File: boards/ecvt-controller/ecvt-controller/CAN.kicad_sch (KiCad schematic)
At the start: 23 parts, among them SW1 SW_SPST, SW2 SW_SPST, U1 TJA1051T-3, U3 MCP2515-xSO, U5 ACT45B-101-2P-TL003, U6 PESD2CAN,215, Y2 ABM3-16.000MHZ-D2Y-T

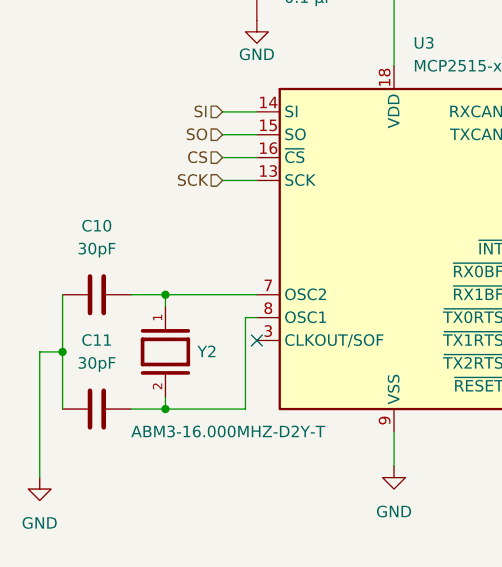
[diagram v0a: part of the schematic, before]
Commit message: ADC done
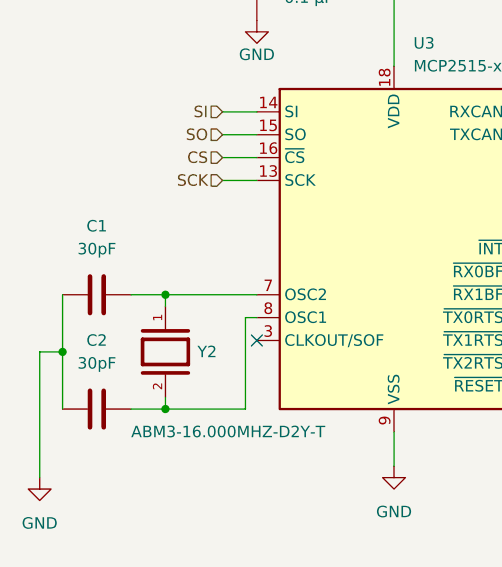
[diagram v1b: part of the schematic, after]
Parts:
- removed C10, C11: 30pF, Capacitor_SMD:C_0805_2012Metric_Pad1.18x1.45mm_HandSolder, symbol Device:C
- added C1, C2: 30pF, Capacitor_SMD:C_0603_1608Metric_Pad1.08x0.95mm_HandSolder, symbol baja-common-parts:C_0603
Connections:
- net GND: now also C1.1, C2.1
- net at U3.7 (OSC2), Y2.1: now also C1.2
- net at U3.8 (OSC1), Y2.2: now also C2.2
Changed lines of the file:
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@@
 			)
 		)
-		(property "Datasheet" ""
+		(property "Datasheet" "file://C:\\Users\\manas\\OneDrive - Northwestern University\\Northwestern\\Extracurricular\\hardware\\libraries\\datasheets\\cmf_automotive_signal_act45b_en.pdf"
 			(at 214.63 97.79 0)
 			(hide yes)
@@
 	)
 	(symbol
-		(lib_id "Device:C")
-		(at 21.59 124.46 90)
-		(unit 1)
-		(body_style 1)
-		(exclude_from_sim no)
-		(in_bom yes)
-		(on_board yes)
-		(in_pos_files yes)
-		(dnp no)
-		(fields_autoplaced yes)
-		(property "Reference" "C11"
-			(at 21.59 116.84 90)
-			(show_name no)
-			(do_not_autoplace no)
-			(effects
-				(font
-					(size 1.27 1.27)
-				)
-			)
-		)
-		(property "Value" "30pF"
-			(at 21.59 119.38 90)
-			(show_name no)
-			(do_not_autoplace no)
-			(effects
-				(font
-					(size 1.27 1.27)
-				)
-			)
-		)
-		(property "Footprint" "Capacitor_SMD:C_0805_2012Metric_Pad1.18x1.45mm_HandSolder"
-			(at 25.4 123.4948 0)
-			(hide yes)
-			(show_name no)
-			(do_not_autoplace no)
-			(effects
-				(font
-					(size 1.27 1.27)
-				)
-			)
-		)
-		(property "Datasheet" ""
-			(at 21.59 124.46 0)
-			(hide yes)
-			(show_name no)
-			(do_not_autoplace no)
-			(effects
-				(font
-					(size 1.27 1.27)
-				)
-			)
-		)
-		(property "Description" "Unpolarized capacitor"
-			(at 21.59 124.46 0)
-			(hide yes)
-			(show_name no)
-			(do_not_autoplace no)
-			(effects
-				(font
-					(size 1.27 1.27)
-				)
-			)
-		)
-		(pin "1"
-		)
-		(pin "2"
-		)
-		(instances
-			(project "ecvt-controller"
-				(path "/6a3c849d-efdf-47ab-8467-b82fc2fbc70f/577f7b7d-9ccb-4072-8b99-2d0e10acd900"
-					(reference "C11")
-					(unit 1)
-				)
-			)
-		)
-	)
-	(symbol
 		(lib_id "power:+3.3V")
 		(at 54.61 66.04 0)
@@
 			)
 		)
-		(property "Datasheet" ""
+		(property "Datasheet" "file://C:\\Users\\manas\\OneDrive - Northwestern University\\Northwestern\\Extracurricular\\hardware\\libraries\\datasheets\\PESD2CANFD24VT-Q.pdf"
 			(at 186.69 91.44 0)
 			(hide yes)
@@
 	)
 	(symbol
+		(lib_id "baja-common-parts:C_0603")
+		(at 21.59 124.46 90)
+		(unit 1)
+		(body_style 1)
+		(exclude_from_sim no)
+		(in_bom yes)
+		(on_board yes)
+		(in_pos_files yes)
+		(dnp no)
+		(fields_autoplaced yes)
+		(property "Reference" "C2"
+			(at 21.59 116.84 90)
+			(show_name no)
+			(do_not_autoplace no)
+			(effects
+				(font
+					(size 1.27 1.27)
+				)
+			)
+		)
+		(property "Value" "30pF"
+			(at 21.59 119.38 90)
+			(show_name no)
+			(do_not_autoplace no)
+			(effects
+				(font
+					(size 1.27 1.27)
+				)
+			)
+		)
+		(property "Footprint" "Capacitor_SMD:C_0603_1608Metric_Pad1.08x0.95mm_HandSolder"
+			(at 24.13 124.46 0)
+			(hide yes)
+			(show_name no)
+			(do_not_autoplace no)
+			(effects
+				(font
+					(size 1.27 1.27)
+				)
+			)
+		)
+		(property "Datasheet" ""
+			(at 26.67 124.46 0)
+			(hide yes)
+			(show_name no)
+			(do_not_autoplace no)
+			(effects
+				(font
+					(size 1.27 1.27)
+				)
+			)
+		)
+		(property "Description" "Capacitor 0603 (1608 metric) HandSolder - Baja default passive size"
+			(at 29.21 124.46 0)
+			(hide yes)
+			(show_name no)
+			(do_not_autoplace no)
+			(effects
+				(font
+					(size 1.27 1.27)
+				)
+			)
+		)
+		(pin "2"
+		)
+		(pin "1"
+		)
+		(instances
+			(project "ecvt-controller"
+				(path "/6a3c849d-efdf-47ab-8467-b82fc2fbc70f/577f7b7d-9ccb-4072-8b99-2d0e10acd900"
+					(reference "C2")
+					(unit 1)
+				)
+			)
+		)
+	)
+	(symbol
 		(lib_id "Device:C")
 		(at 269.24 123.19 0)
@@
 				(path "/6a3c849d-efdf-47ab-8467-b82fc2fbc70f/577f7b7d-9ccb-4072-8b99-2d0e10acd900"
 					(reference "#PWR049")
-					(unit 1)
-				)
-			)
-		)
-	)
-	(symbol
-		(lib_id "Device:C")
-		(at 21.59 111.76 90)
-		(unit 1)
-		(body_style 1)
-		(exclude_from_sim no)
-		(in_bom yes)
-		(on_board yes)
-		(in_pos_files yes)
-		(dnp no)
-		(fields_autoplaced yes)
-		(property "Reference" "C10"
-			(at 21.59 104.14 90)
-			(show_name no)
-			(do_not_autoplace no)
-			(effects
-				(font
-					(size 1.27 1.27)
-				)
-			)
-		)
-		(property "Value" "30pF"
-			(at 21.59 106.68 90)
-			(show_name no)
-			(do_not_autoplace no)
-			(effects
-				(font
-					(size 1.27 1.27)
-				)
-			)
-		)
-		(property "Footprint" "Capacitor_SMD:C_0805_2012Metric_Pad1.18x1.45mm_HandSolder"
-			(at 25.4 110.7948 0)
-			(hide yes)
-			(show_name no)
-			(do_not_autoplace no)
-			(effects
-				(font
-					(size 1.27 1.27)
-				)
-			)
-		)
-		(property "Datasheet" ""
-			(at 21.59 111.76 0)
-			(hide yes)
-			(show_name no)
-			(do_not_autoplace no)
-			(effects
-				(font
-					(size 1.27 1.27)
-				)
-			)
-		)
-		(property "Description" "Unpolarized capacitor"
-			(at 21.59 111.76 0)
-			(hide yes)
-			(show_name no)
-			(do_not_autoplace no)
-			(effects
-				(font
-					(size 1.27 1.27)
-				)
-			)
-		)
-		(pin "1"
-		)
-		(pin "2"
-		)
-		(instances
-			(project "ecvt-controller"
-				(path "/6a3c849d-efdf-47ab-8467-b82fc2fbc70f/577f7b7d-9ccb-4072-8b99-2d0e10acd900"
-					(reference "C10")
 					(unit 1)
 				)
@@
 					(unit 1)
 				)
+			)
+		)
+	)
+	(symbol
+		(lib_id "baja-common-parts:C_0603")
+		(at 21.59 111.76 90)
+		(unit 1)
+		(body_style 1)
+		(exclude_from_sim no)
+		(in_bom yes)
+		(on_board yes)
+		(in_pos_files yes)
+		(dnp no)
+		(fields_autoplaced yes)
+		(property "Reference" "C1"
+			(at 21.59 104.14 90)
+			(show_name no)
+			(do_not_autoplace no)
+			(effects
+				(font
+					(size 1.27 1.27)
+				)
+			)
+		)
+		(property "Value" "30pF"
+			(at 21.59 106.68 90)
+			(show_name no)
+			(do_not_autoplace no)
+			(effects
+				(font
+					(size 1.27 1.27)
+				)
+			)
+		)
+		(property "Footprint" "Capacitor_SMD:C_0603_1608Metric_Pad1.08x0.95mm_HandSolder"
+			(at 24.13 111.76 0)
+			(hide yes)
+			(show_name no)
+			(do_not_autoplace no)
+			(effects
+				(font
+					(size 1.27 1.27)
+				)
+			)
+		)
+		(property "Datasheet" ""
+			(at 26.67 111.76 0)
+			(hide yes)
+			(show_name no)
+			(do_not_autoplace no)
+			(effects
+				(font
+					(size 1.27 1.27)
+				)
+			)
+		)
+		(property "Description" "Capacitor 0603 (1608 metric) HandSolder - Baja default passive size"
+			(at 29.21 111.76 0)
+			(hide yes)
+			(show_name no)
+			(do_not_autoplace no)
+			(effects
+				(font
+					(size 1.27 1.27)
+				)
+			)
+		)
+		(pin "2"
+		)
+		(pin "1"
+		)
+		(instances
+			(project "ecvt-controller"
+				(path "/6a3c849d-efdf-47ab-8467-b82fc2fbc70f/577f7b7d-9ccb-4072-8b99-2d0e10acd900"
+					(reference "C1")
+					(unit 1)
+				)
